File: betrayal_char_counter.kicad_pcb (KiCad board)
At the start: 2 copper layers, 123.2 x 118.1 mm, 61 parts, among them J1 AVR-ISP-6, SW1 SW_ON, SW10 SW_Push, SW2 SW_Push, SW3 SW_Push, SW4 SW_Push, SW5 SW_Push, SW6 SW_Push, SW7 SW_Push, SW8 SW_Push, SW9 SW_Push, U1 MCP1640CH, U2 ATtiny88-AU

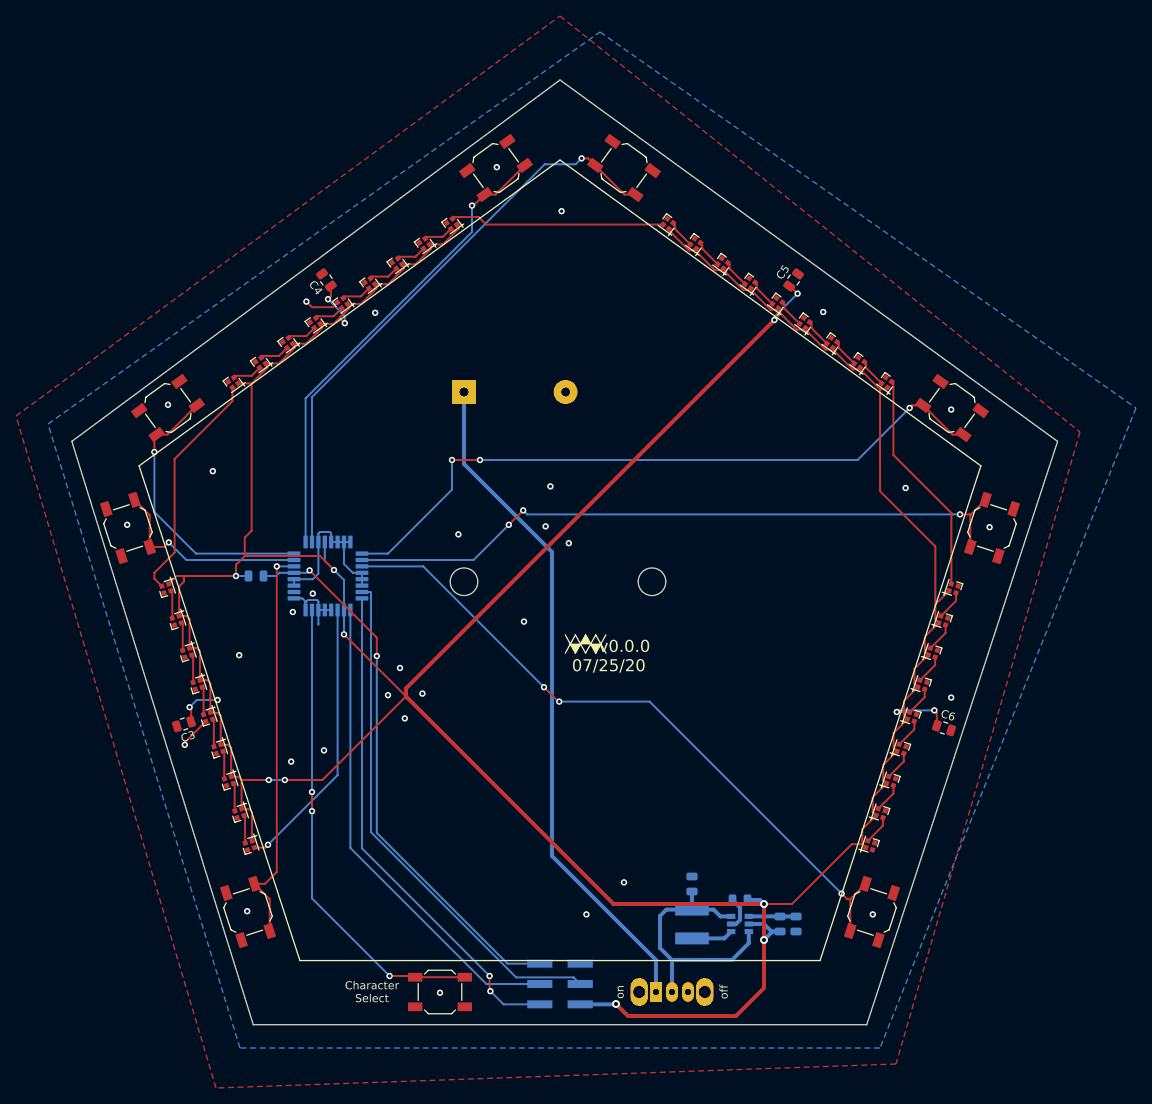
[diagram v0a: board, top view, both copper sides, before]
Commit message: Add 1mm height
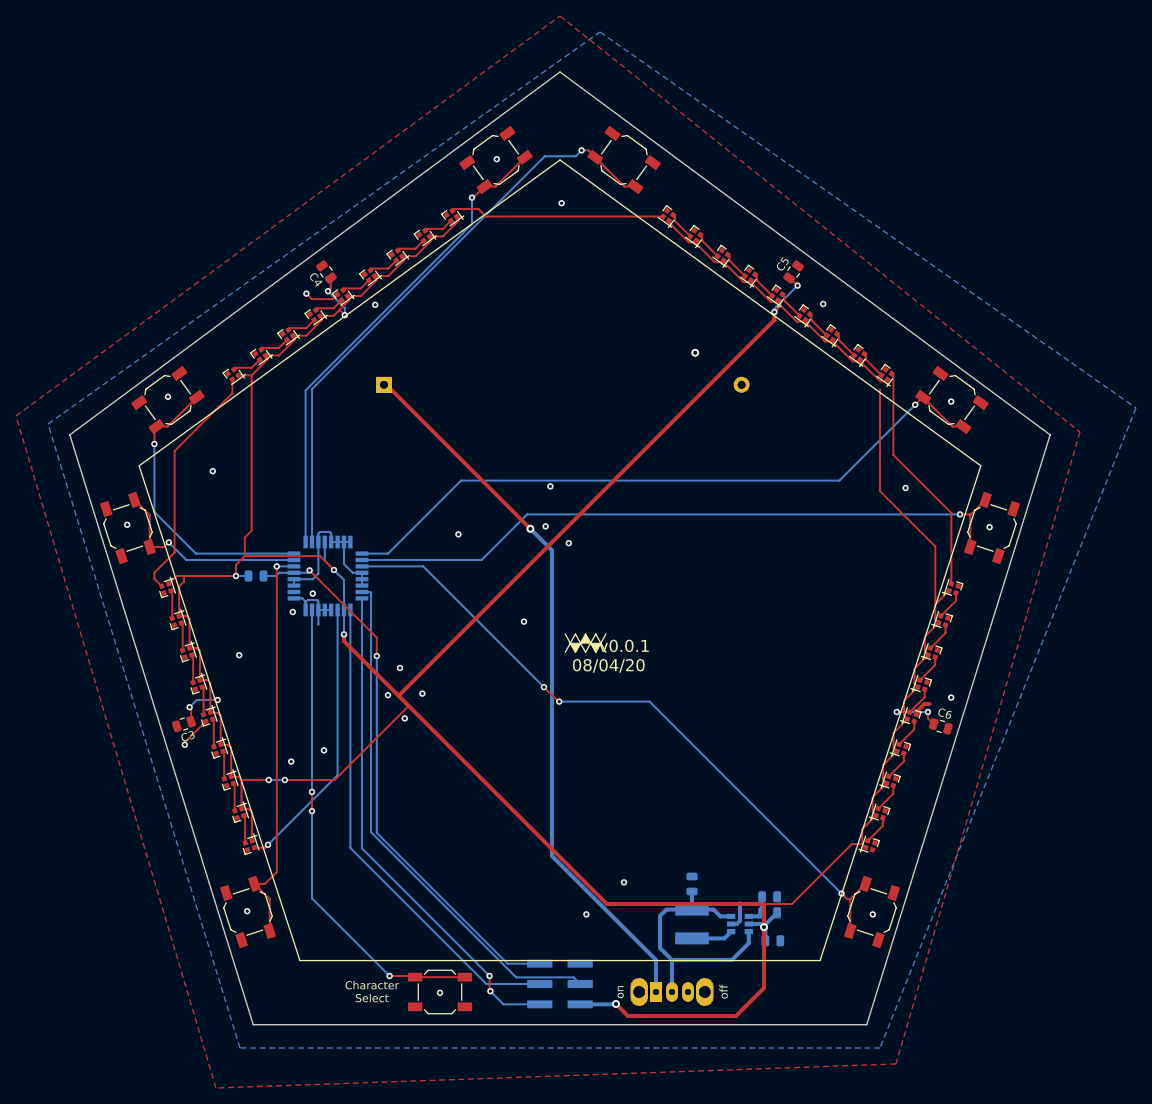
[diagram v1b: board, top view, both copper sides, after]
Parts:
- BT1: value 3xAAA -> 1xAAA; footprint Battery:BatteryHolder_Keystone_2479_3xAAA -> Battery:BatteryHolder_Keystone_2466_1xAAA
- moved BT1 10.0 mm to (78.0, 68.1), turned to 0 degrees
- moved C2 6.54 mm to (126.6, 137.6), turned to 0 degrees
- moved R2 4.74 mm to (126.2, 132.1), turned to 0 degrees
- moved R1 1.91 mm to (126.2, 134.1), turned to 0 degrees
- moved C4 1.00 mm to (70.8, 54.0)
- moved C5 1.00 mm to (129.2, 54.0)
- moved D10 1.00 mm to (59.1, 66.8)
- moved D11 1.00 mm to (62.6, 64.3)
- moved D12 1.00 mm to (66.0, 61.9)
- moved D13 1.00 mm to (69.4, 59.4)
- moved D14 1.00 mm to (72.8, 56.9)
- moved D15 1.00 mm to (76.2, 54.4)
- moved D16 1.00 mm to (79.6, 51.9)
- moved D17 1.00 mm to (83.0, 49.5)
- moved D18 1.00 mm to (86.5, 47.0)
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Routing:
- net Net-(BT1-Pad1): track 84.9 -> 90.2 mm, vias 0 -> 1
- net Net-(R1-Pad1): track 5.91 -> 3.85 mm
- net SN_DN: track 86.5 -> 84.8 mm, vias 3 -> 1
- net GND: track 44.0 -> 45.6 mm, vias 32 -> 33
- net SN_UP: track 72.8 -> 73.8 mm
- net MI_UP: track 59.3 -> 60.3 mm
- net MI_DN: track 35.9 -> 36.9 mm
- net /StatTrack_Might/DIN: track 29.2 -> 30.2 mm
- net /StatTrack_Knowledge/DIN: track 28.4 -> 29.4 mm
- net KN_UP: track 85.5 -> 85.1 mm, vias 3 -> 1
- net 5V: track 492.8 -> 493.1 mm, vias 16 -> 15
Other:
- board size 123.2 x 118.1 mm -> 122.5 x 119.1 mm
- board text added: "v0.0.1 08/04/20"
- board text removed: "v0.0.0 07/25/20"
